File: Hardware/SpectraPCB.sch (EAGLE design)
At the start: 49 parts, among them IC1 L293D, J1 POWER_JACK, Q1 8/16/20MHz, U1 MCP73831, U2 MAX1704X, U3 MIC5205, U4 ATMEGA328

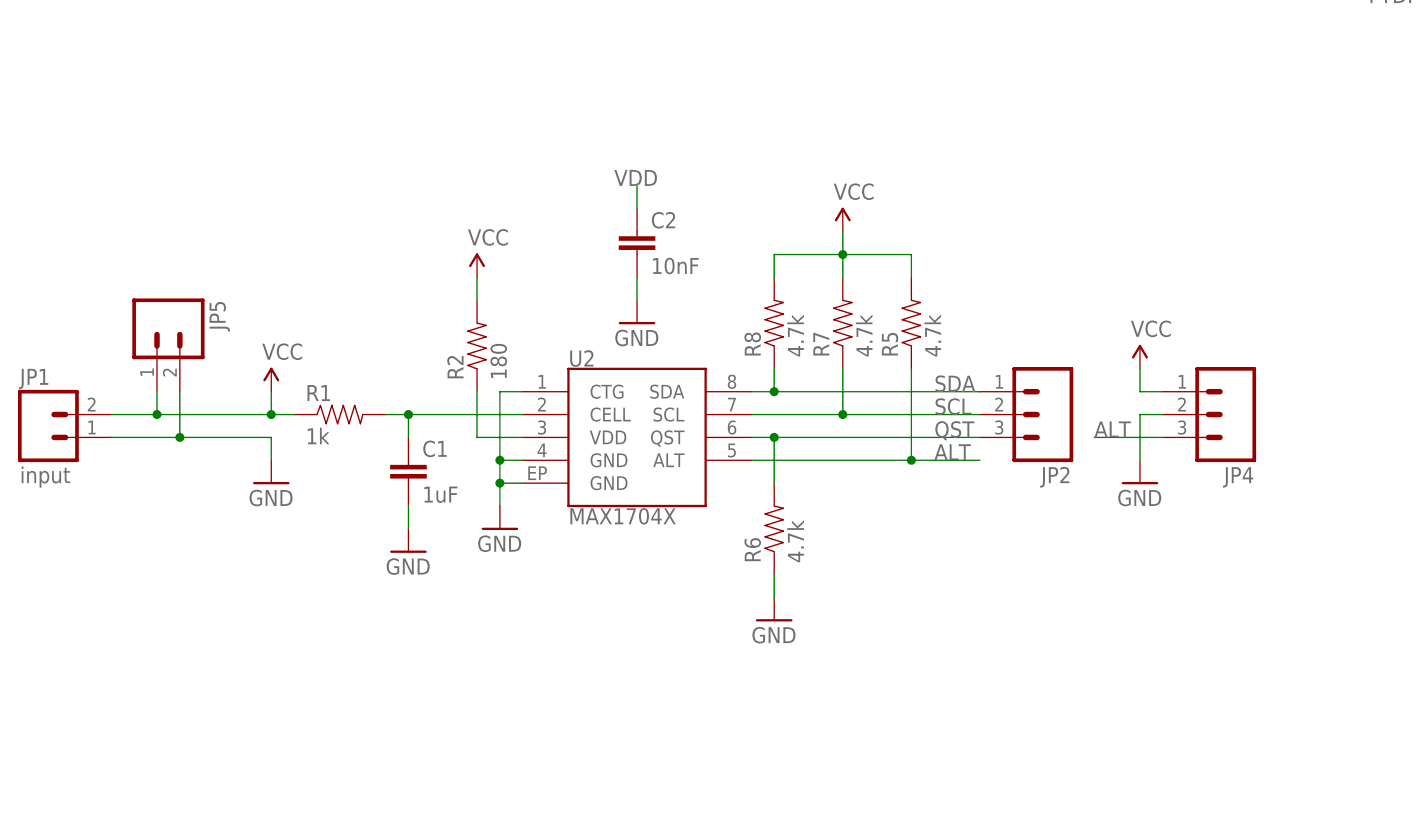
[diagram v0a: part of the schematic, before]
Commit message: updates
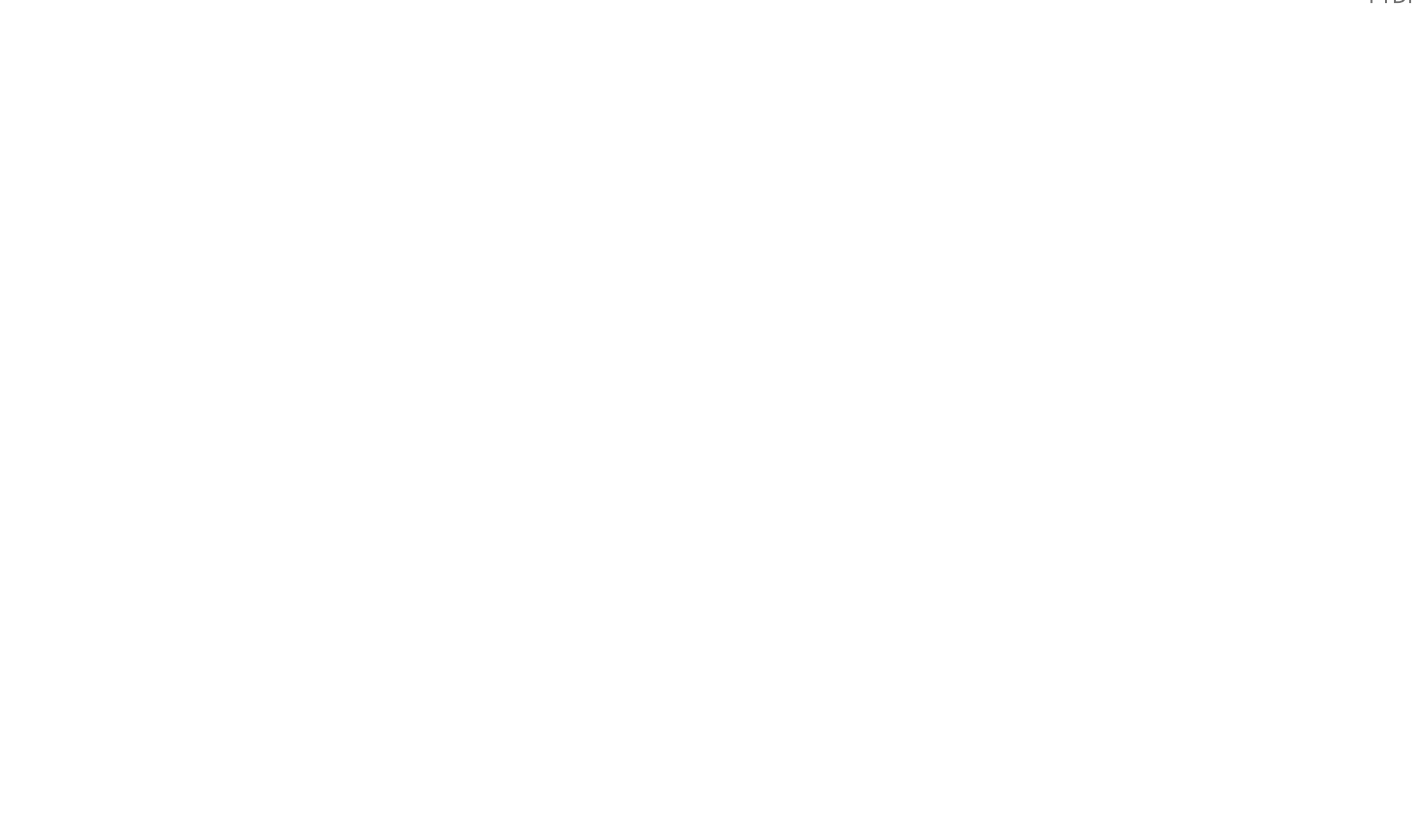
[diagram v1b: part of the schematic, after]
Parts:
- removed C1: 1uF, SparkFun:CAP0402-CAP
- removed C2: 10nF, SparkFun:CAP0402-CAP
- removed JP1: input, SparkFun:M02-JST-2MM-SMT
- removed JP2, JP4: (no value), SparkFun:M03PTH
- removed JP5: (no value), SparkFun:M02PTH
- removed R1: 1k, SparkFun:RESISTOR0402-RES
- removed R2: 180, SparkFun:RESISTOR0402-RES
- removed R5, R6, R7, R8: 4.7k, SparkFun:RESISTOR0402-RES
- removed U2: MAX1704X, SparkFun:MAX1704X
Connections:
- removed net ALT: JP4.3, R5.1, U2.ALT
- removed net N$2: C1.1, R1.2, U2.CELL
- removed net QST: JP2.3, R6.2, U2.QST
- removed net SCL: JP2.2, R7.1, U2.SCL
- removed net SDA: JP2.1, R8.1, U2.SDA
- removed net VDD: C2.1, R2.1, U2.VDD
- net GND: no longer C1.2, C2.2, JP1.1, JP4.2, JP5.2, R6.1, U2.CTG, U2.GND@4, U2.GND@EP
- net VCC: no longer JP1.2, JP4.1, JP5.1, R1.1, R2.2, R5.2, R7.2, R8.2

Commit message: adding all the design blocks
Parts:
- removed C3, C4: 4.7uF, SparkFun:CAP0402-CAP
- removed D11: RED, SparkFun:LED0603
- removed IC1: L293D, st-microelectronics:L293D
- removed J1: POWER_JACK, SparkFun-Connectors:POWER_JACK
- removed JP7: LiPo Battery, SparkFun:M02-JST-2MM-SMT
- removed JP8: (no value), SparkFun:M02PTH
- removed U1: MCP73831, SparkFun:MCP73831
- added AMT103-V: PURDUE-EWH-ENCODER, Purdue-EWH-Encoder:PURDUE-EWH-ENCODER
- added C1: (no value), resistor:C-EUC0603
- added C2: (no value), resistor:C-EUC0402
- added C8, C9: 4.7uF, SparkFun:CAP0402-CAP
- added D1: RED, SparkFun:LED0603
- added IC2: L293D, st-microelectronics:L293D
- added IC3: MCP601OT, CalvEngIO-AnalogIC:MCP601OT
- added J2: POWER_JACK, SparkFun-Connectors:POWER_JACK
- added JP1: LiPo Battery, SparkFun:M02-JST-2MM-SMT
- added JP2: (no value), SparkFun:M02PTH
- added R1, R2, R5, R6: 10k, SparkFun-Resistors:10KOHM-0603-1/10W-1%
- added R7: 330, SparkFun:RESISTOR0402-RES
- added R8: 2K, SparkFun:RESISTOR0402-RES
- added U$1: EWH_KEYPAD, Purdue-EWH-Keypad:EWH_KEYPAD
- added U2: MCP73831, SparkFun:MCP73831
- R3: value 330 -> (none); device SparkFun:RESISTOR0402-RES -> resistor:R-US_R0402
- R4: value 2K -> (none); device SparkFun:RESISTOR0402-RES -> resistor:R-US_R0402
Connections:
- removed net PROG: R4.1, U1.PROG
- removed net STAT: D11.C, U1.STAT
- new net 5V: AMT103-V.SW+, IC2.1-2EN, IC2.3-4EN, IC3.V+, R3.2
- new net D11: AMT103-V.B
- new net N$10: U$1.D9
- new net N$11: R1.2, U$1.D8
- new net N$12: U$1.D7
- new net N$13: R2.2, U$1.D6
- new net N$14: R6.2, U$1.D4
- new net N$15: R1.1, R2.1, R5.1, R6.1
- new net N$16: R5.2, U$1.D5
- new net N$17: D1.A, R7.1
- new net N$18: IC3.-IN, IC3.OUT
- new net N$2: C1.1, IC2.VCC2
- new net N$8: C2.1, IC2.VCC1
- new net N$9: U$1.D10
- new net PROG1: R8.1, U2.PROG
- new net STAT1: D1.C, U2.STAT
- new net STEPPER_ROB-10846: IC2.1Y, IC2.2Y, IC2.3Y, IC2.4Y
- net A0: now also IC2.1A
- net A1: now also IC2.2A
- net A2: now also IC2.4A
- net A3: now also IC2.3A
- net CHRG.CTRL: now also R8.2; no longer R4.2
- net D3: now also AMT103-V.A
- net GND: now also AMT103-V.SW-, C1.2, C8.2, C9.2, IC2.GND1, IC2.GND2, IC2.GND3, IC2.GND4, IC3.V-, J2.GND, J2.GNDBREAK, JP1.1, JP2.1, R4.1, U2.VSS; no longer C3.2, C4.2, JP7.1, JP8.1, U1.VSS
- net N$3: now also IC3.+IN, R4.2; no longer D11.A
- net VCC: now also C9.1, JP1.2, JP2.2, U2.VBAT; no longer C4.1, JP7.2, JP8.2, U1.VBAT
- net VIN: now also C8.1, J2.PWR, R7.2, U2.VIN; no longer C3.1, R3.2, U1.VIN
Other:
- note added: "#"
- note added: "*"
- note added: "0"
- note added: "1"
- note added: "2"
- note added: "3"
- note added: "4"
- note added: "5"
- note added: "6"
- note added: "7"
- note added: "8"
- note added: "9"
- note added: "<KEYPAD COM-08653"
- moved on the sheet: R3, R4
